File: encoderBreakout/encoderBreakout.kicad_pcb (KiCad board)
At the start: 2 copper layers, 49.5 x 51.5 mm, 2 parts, among them J1 Conn_01x08_MountingPin

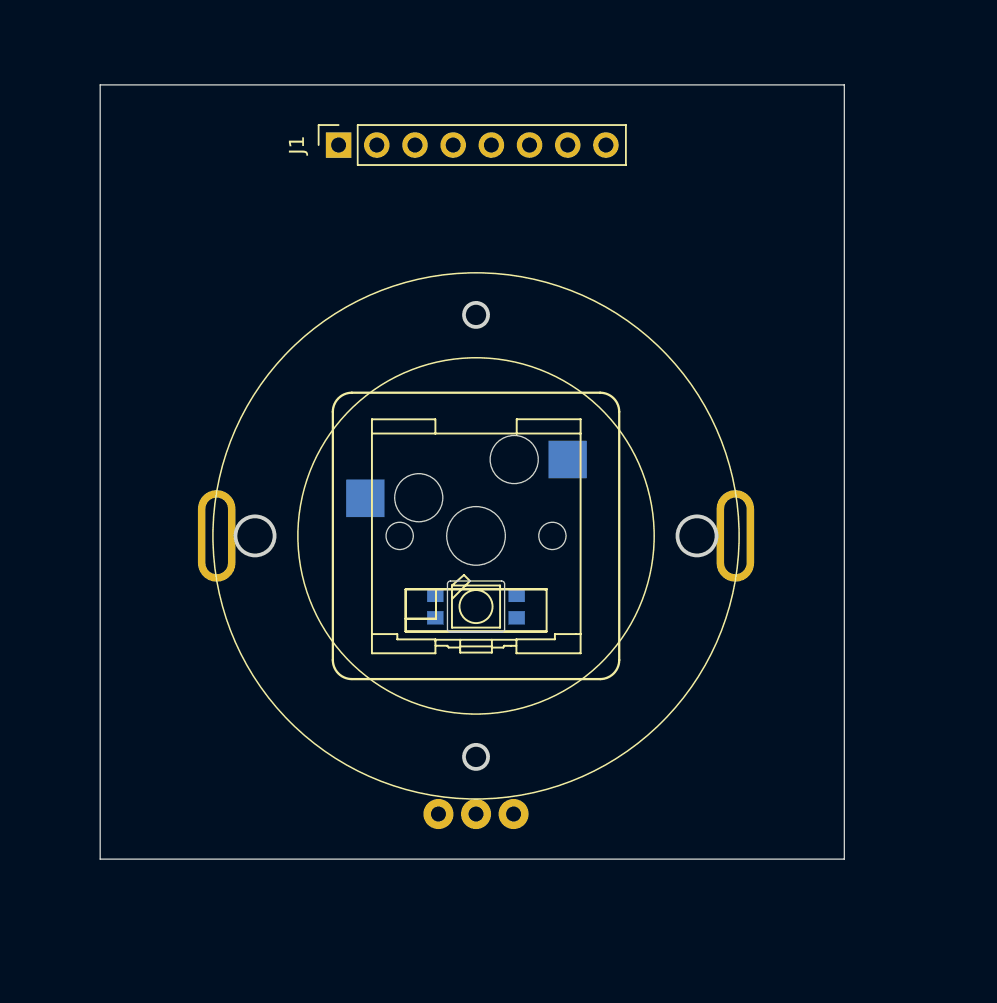
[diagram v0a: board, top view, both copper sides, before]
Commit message: encoder breakout rev a
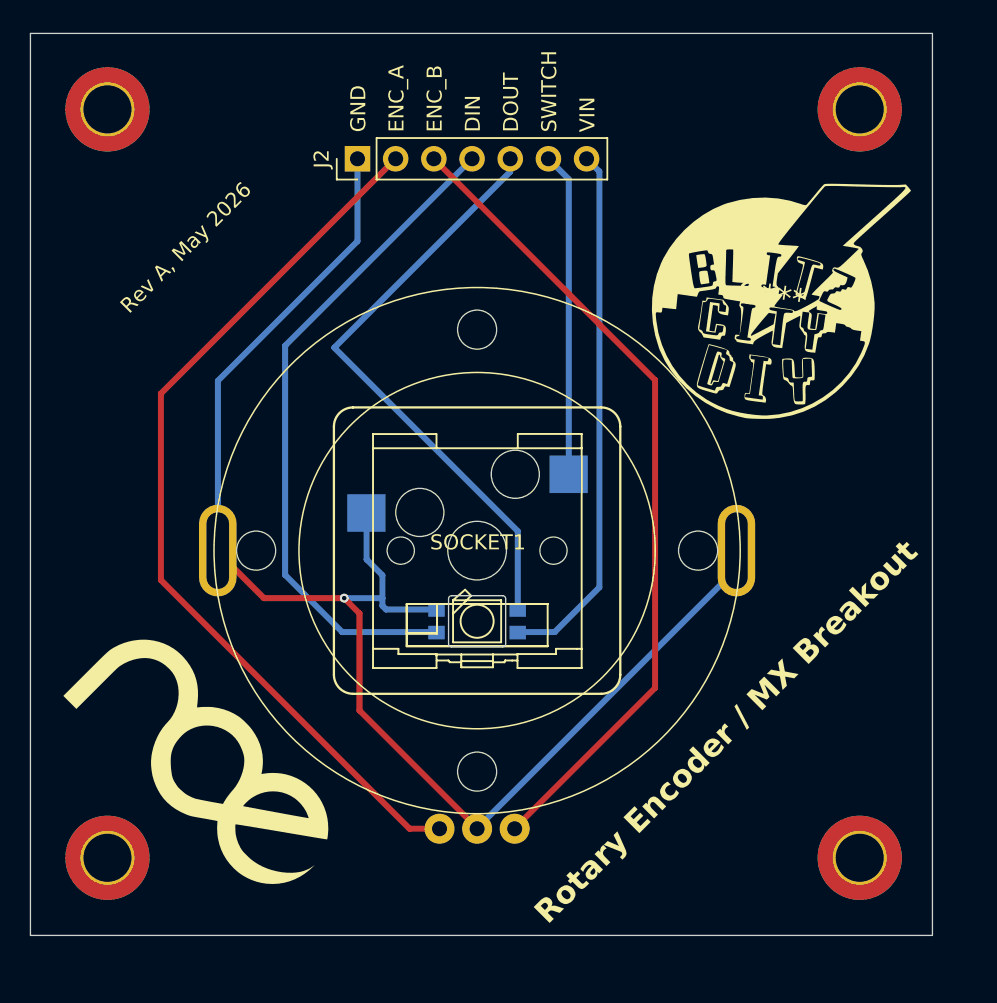
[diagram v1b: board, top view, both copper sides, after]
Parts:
- removed J1: Conn_01x08_MountingPin, Connector_PinSocket_2.54mm:PinSocket_1x08_P2.54mm_Vertical
- removed encoderWithKailh1: ~, encLibrary:EC35AwithKailhSocket
- added ENC1: ~, blitz_lib:EC35A_nosocket, F.Cu at (150.6, 101.0)
- added G***: LOGO, LOGO, F.Cu at (170.2, 84.1)
- added G***: LOGO, LOGO, F.Cu at (132.6, 115.1)
- added J2: Conn_01x07_Pin, Connector_PinHeader_2.54mm:PinHeader_1x07_P2.54mm_Vertical, F.Cu at (142.6, 74.9)
- added REF**: MountingHole_3.2mm_M3_DIN965_Pad_TopBottom, MountingHole:MountingHole_3.2mm_M3_DIN965_Pad_TopBottom, F.Cu at (126.0, 71.6)
- added REF**: MountingHole_3.2mm_M3_DIN965_Pad_TopBottom, MountingHole:MountingHole_3.2mm_M3_DIN965_Pad_TopBottom, F.Cu at (176.0, 71.6)
- added REF**: MountingHole_3.2mm_M3_DIN965_Pad_TopBottom, MountingHole:MountingHole_3.2mm_M3_DIN965_Pad_TopBottom, F.Cu at (176.0, 121.4)
- added REF**: MountingHole_3.2mm_M3_DIN965_Pad_TopBottom, MountingHole:MountingHole_3.2mm_M3_DIN965_Pad_TopBottom, F.Cu at (126.0, 121.4)
- added REV_NEOPIXEL1: ~, blitz_lib:reverse_neopixel, F.Cu at (150.6, 101.0)
- added SOCKET1: ~, blitz_lib:kailh_socket, F.Cu at (150.6, 101.0)
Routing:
- net GND: track 0.00 -> 99.0 mm, vias 0 -> 1
- net /ENC_A: track 0.00 -> 59.9 mm
- net /ENC_B: track 0.00 -> 54.5 mm
- net /NEO_DIN: track 0.00 -> 44.5 mm
- net /NEO_DOUT: track 0.00 -> 39.9 mm
- net +3.3V: track 0.00 -> 35.5 mm
- net /SWITCH: track 0.00 -> 21.5 mm
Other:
- board size 49.5 x 51.5 mm -> 60 x 60 mm
- board text added: "DIN"
- board text added: "DOUT"
- board text added: "ENC_A"
- board text added: "ENC_B"
- board text added: "GND"
- board text added: "Rev A, May 2026"
- board text added: "Rotary Encoder / MX Breakout"
- board text added: "SWITCH"
- board text added: "VIN"
